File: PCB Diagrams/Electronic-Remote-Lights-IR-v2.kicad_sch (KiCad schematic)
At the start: 16 parts, among them J1 POWER, J2 220V, K1 RELAY, SW1 RESET, U1 VS1338B

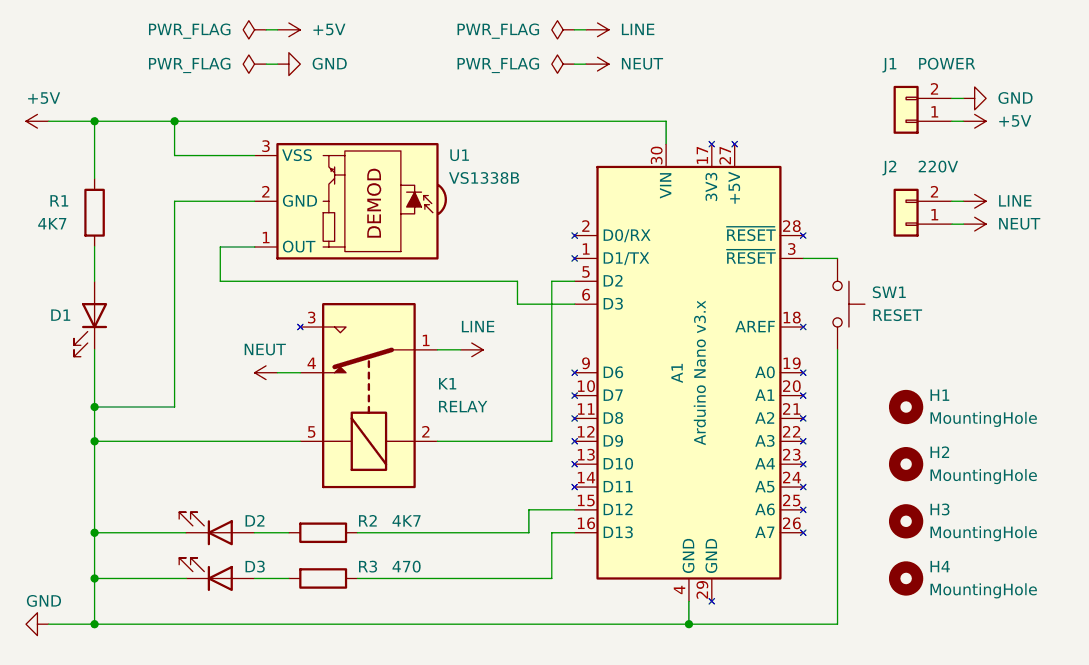
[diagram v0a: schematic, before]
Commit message: PCB bug fix
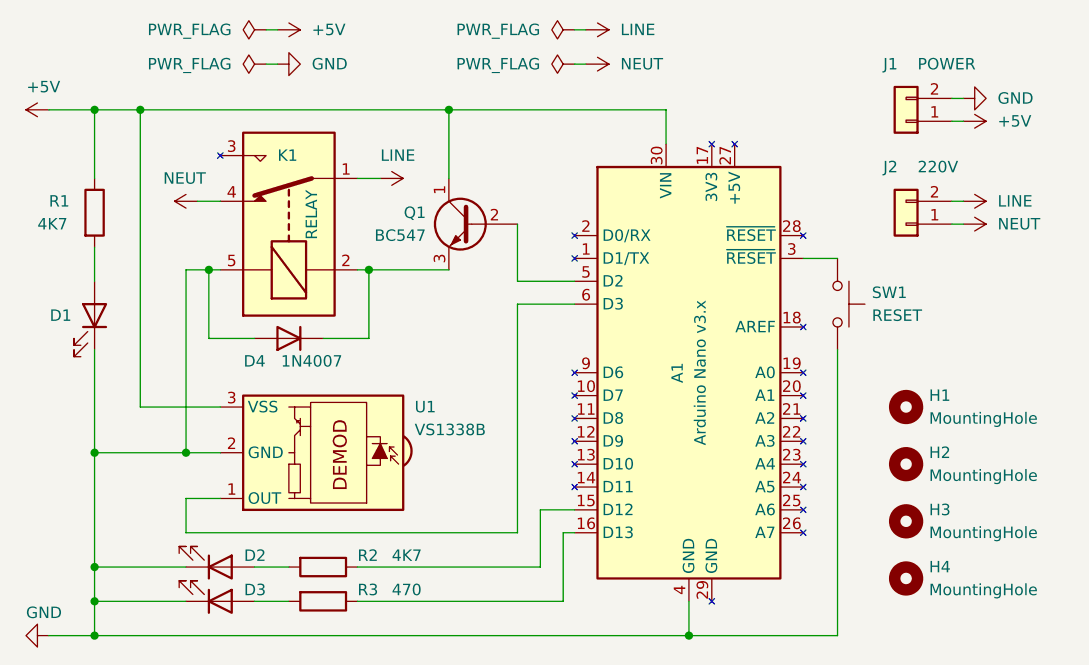
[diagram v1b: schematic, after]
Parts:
- added D4: 1N4007, Diode_THT:D_DO-41_SOD81_P10.16mm_Horizontal, symbol Diode:1N4007
- added Q1: BC547, Package_TO_SOT_THT:TO-92_Inline_Wide, symbol Transistor_BJT:BC547
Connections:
- net +5V: now also Q1.1 (C)
- net GND: now also D4.2 (A)
- net at A1.5 (D2): now also Q1.2 (B); no longer K1.2
- new net: D4.1 (K), K1.2, Q1.3 (E)
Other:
- moved on the sheet: D2, D3, K1, R2, R3, U1
